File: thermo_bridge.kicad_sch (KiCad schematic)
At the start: 4 parts

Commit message: fields
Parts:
- R3301, R3302, R3303, R3304: gfootprint 0603 -> (none)
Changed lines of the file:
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@@
-			)
-		)
-		(property "gfootprint" "0603"
-			(at 184.15 3.81 0)
-			(effects
-				(font
-					(size 1.27 1.27)
-				)
-				(hide yes)
 			)
 		)
@@
 			)
 		)
-		(property "gfootprint" "0603"
-			(at 177.8 177.8 0)
-			(effects
-				(font
-					(size 1.27 1.27)
-				)
-				(hide yes)
-			)
-		)
 		(pin "1"
 		)
@@
 			)
 		)
-		(property "gfootprint" "0603"
-			(at 185.42 185.42 0)
-			(effects
-				(font
-					(size 1.27 1.27)
-				)
-				(hide yes)
-			)
-		)
 		(pin "1"
 		)
@@
 			(effects
 				(font
-					(size 1.27 1.27)
-				)
-				(hide yes)
-			)
-		)
-		(property "gfootprint" "0603"
-			(at 191.77 -3.81 0)
-			(effects
-				(font

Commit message: vendor info
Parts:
- R3301, R3304: Vendor (none) -> digikey:490-4800-1-ND
- R3302, R3303: Vendor (none) -> digikey:MCT0603-10K-MDCT-ND
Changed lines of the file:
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@@
+			)
+		)
+		(property "Vendor" "digikey:MCT0603-10K-MDCT-ND"
+			(at 184.15 3.81 0)
+			(effects
+				(font
+					(size 1.27 1.27)
+				)
+				(hide yes)
 			)
 		)
@@
 			)
 		)
+		(property "Vendor" "digikey:490-4800-1-ND"
+			(at 177.8 177.8 0)
+			(effects
+				(font
+					(size 1.27 1.27)
+				)
+				(hide yes)
+			)
+		)
 		(pin "1"
 		)
@@
 			)
 		)
+		(property "Vendor" "digikey:MCT0603-10K-MDCT-ND"
+			(at 185.42 185.42 0)
+			(effects
+				(font
+					(size 1.27 1.27)
+				)
+				(hide yes)
+			)
+		)
 		(pin "1"
 		)
@@
 			(effects
 				(font
+					(size 1.27 1.27)
+				)
+				(hide yes)
+			)
+		)
+		(property "Vendor" "digikey:490-4800-1-ND"
+			(at 191.77 -3.81 0)
+			(effects
+				(font

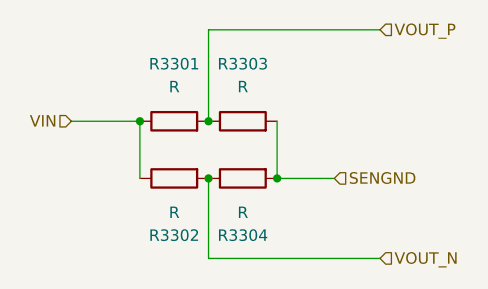
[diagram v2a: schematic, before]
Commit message: update value
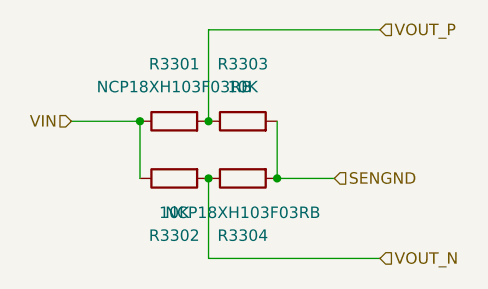
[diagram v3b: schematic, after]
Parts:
- R3301, R3304: value R -> NCP18XH103F03RB
- R3302, R3303: value R -> 10K
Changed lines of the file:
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@@
 			)
 		)
-		(property "Value" "R"
+		(property "Value" "10K"
 			(at 90.17 97.79 90)
 			(effects
@@
 			)
 		)
-		(property "Value" "R"
+		(property "Value" "NCP18XH103F03RB"
 			(at 90.17 83.82 90)
 			(effects
@@
 			)
 		)
-		(property "Value" "R"
+		(property "Value" "10K"
 			(at 97.79 83.82 90)
 			(effects
@@
 			)
 		)
-		(property "Value" "R"
+		(property "Value" "NCP18XH103F03RB"
 			(at 97.79 97.79 90)
 			(effects
